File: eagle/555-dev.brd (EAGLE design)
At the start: 50 x 50 mm, 26 parts, among them IC1 NE555, Q1 IRF740, T1 2N2222

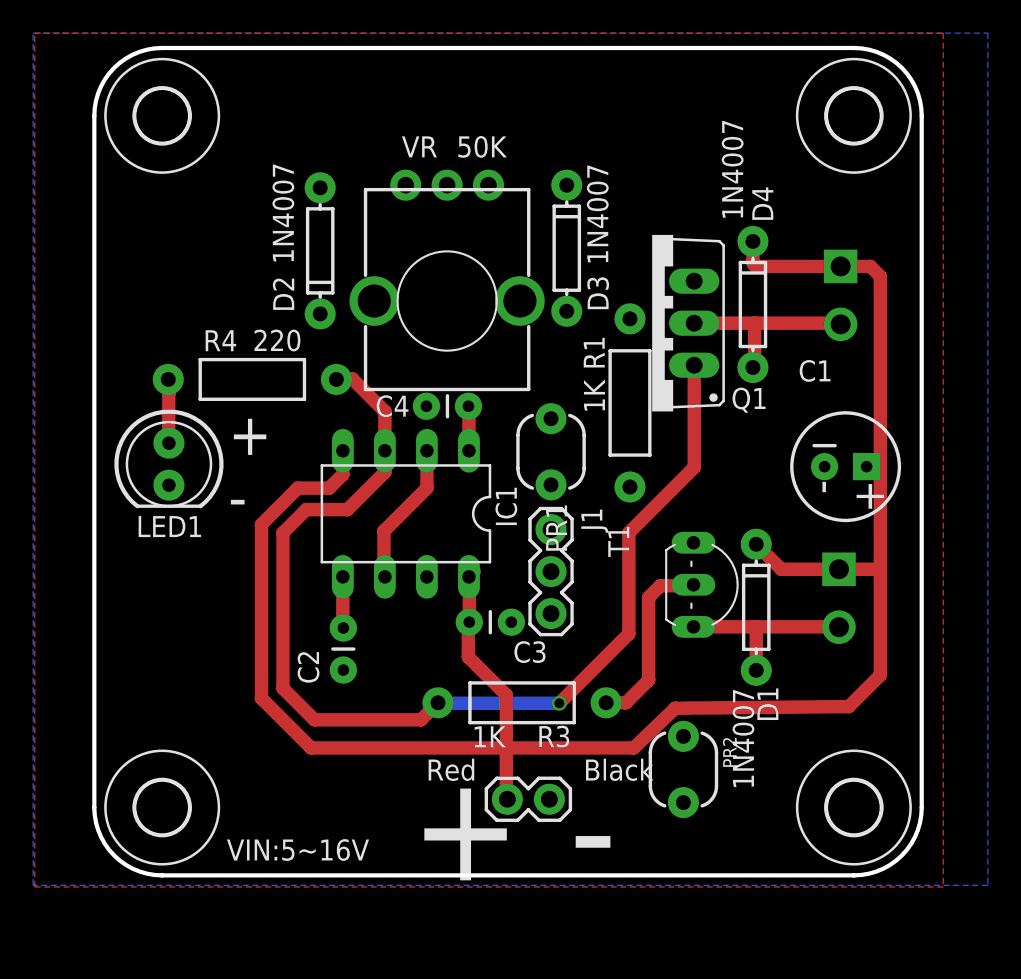
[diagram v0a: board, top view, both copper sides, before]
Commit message: added LOGO
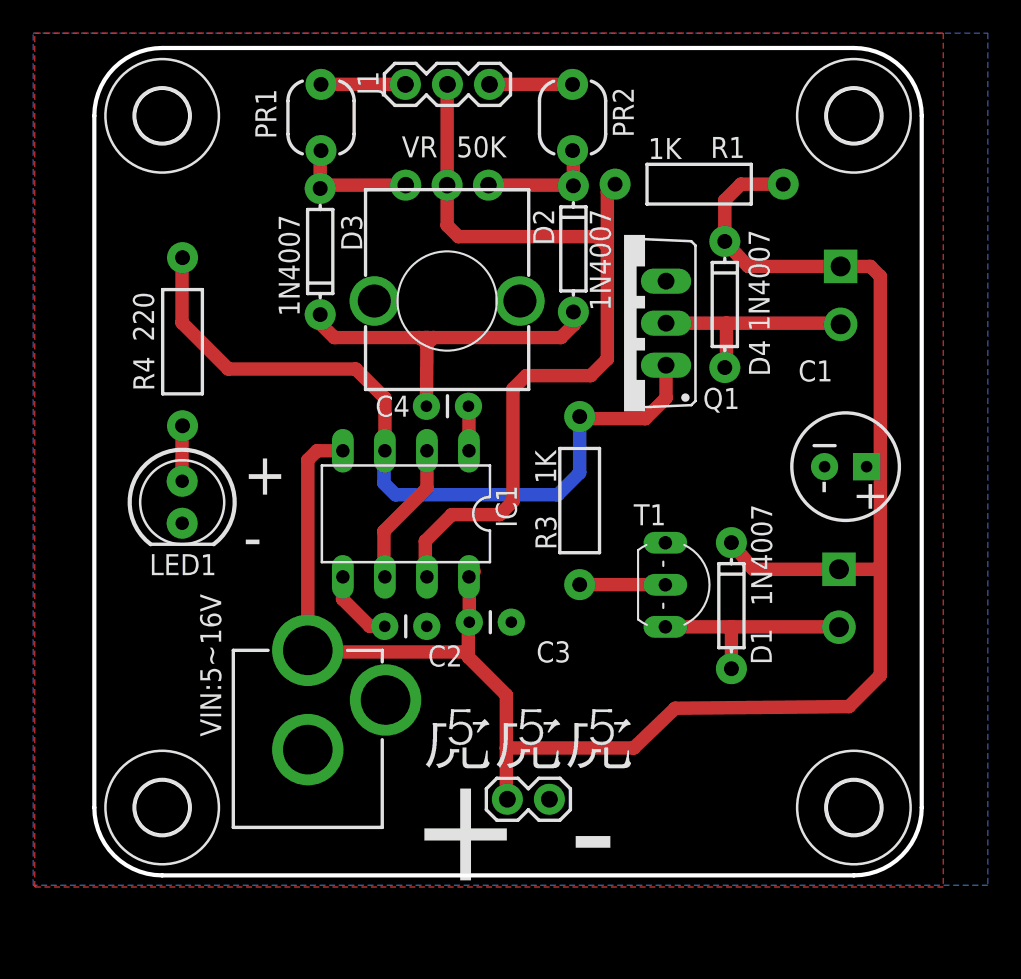
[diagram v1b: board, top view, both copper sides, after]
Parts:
- added JP3: POWER_JACKPTH, SparkFun-Connectors:POWER_JACK_PTH
- added U$1: LOGO, SparkFun-Electromechanical:LOGO
- moved PR2 40.0 mm to (28.9, 45.8), turned to 90 degrees
- moved J1 28.3 mm to (18.8, 47.8), turned to 0 degrees
- moved PR1 24.5 mm to (13.7, 45.8), turned to 90 degrees
- moved D2 15.3 mm to (28.9, 37.9), turned to 90 degrees
- moved D3 14.9 mm to (13.7, 37.7), turned to 270 degrees
- moved R1 13.9 mm to (36.5, 41.8), turned to 0 degrees
- moved R3 12.7 mm to (29.3, 22.6), turned to 90 degrees
- moved R4 4.80 mm to (5.33, 32.2), turned to 90 degrees
- moved C2 2.50 mm to (17.6, 15.1), turned to 0 degrees
- moved LED1 2.44 mm to (5.31, 22.6)
- moved Q1 1.70 mm to (32.0, 33.4)
- moved D4 1.70 mm to (38.1, 34.5)
- moved T1 1.70 mm to (35.8, 17.6)
- moved D1 1.50 mm to (38.5, 16.3)
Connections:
- net GND: now also JP3.GND
- net VCC: now also JP3.PWR
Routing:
- net 555_DISCH: track 0.00 -> 51.8 mm
- net N$4: track 0.00 -> 22.5 mm
- net OUT: track 66.2 -> 47.1 mm, vias 1 -> 0
- net N$2: track 0.00 -> 7.78 mm
- net N$3: track 0.00 -> 7.56 mm
- net N$7: track 11.2 -> 5.18 mm
- net PR1: track 0.00 -> 5.10 mm
- net PR2: track 0.00 -> 5.02 mm
- net LOAD2-: track 11.6 -> 13.3 mm
- net LOAD1-: track 11.4 -> 13.0 mm
- net VCC: track 116.5 -> 115.0 mm
- net N$5: track 3.10 -> 4.58 mm
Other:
- board text removed: "Black"
- board text removed: "Red"
